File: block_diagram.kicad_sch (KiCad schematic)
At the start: 0 parts

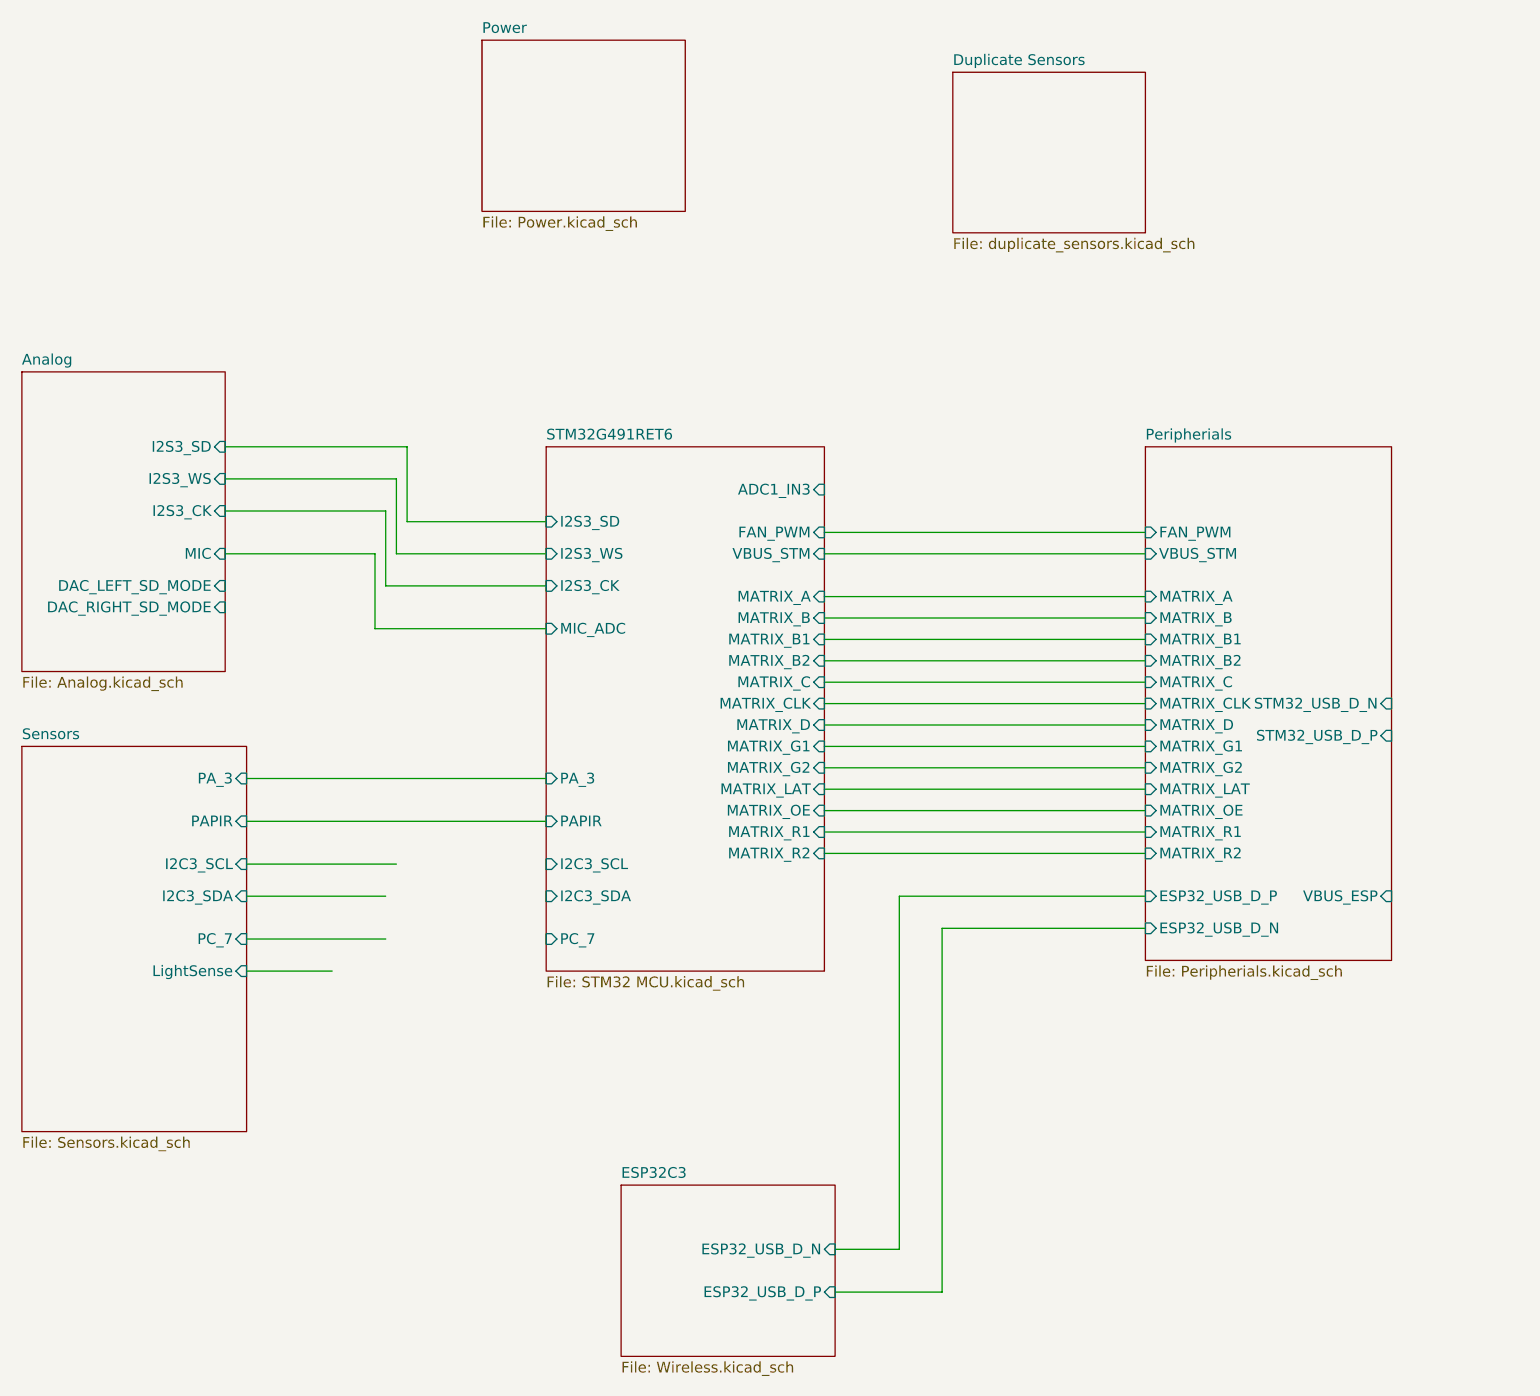
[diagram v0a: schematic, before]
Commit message: Major Changes - Schematic Done??
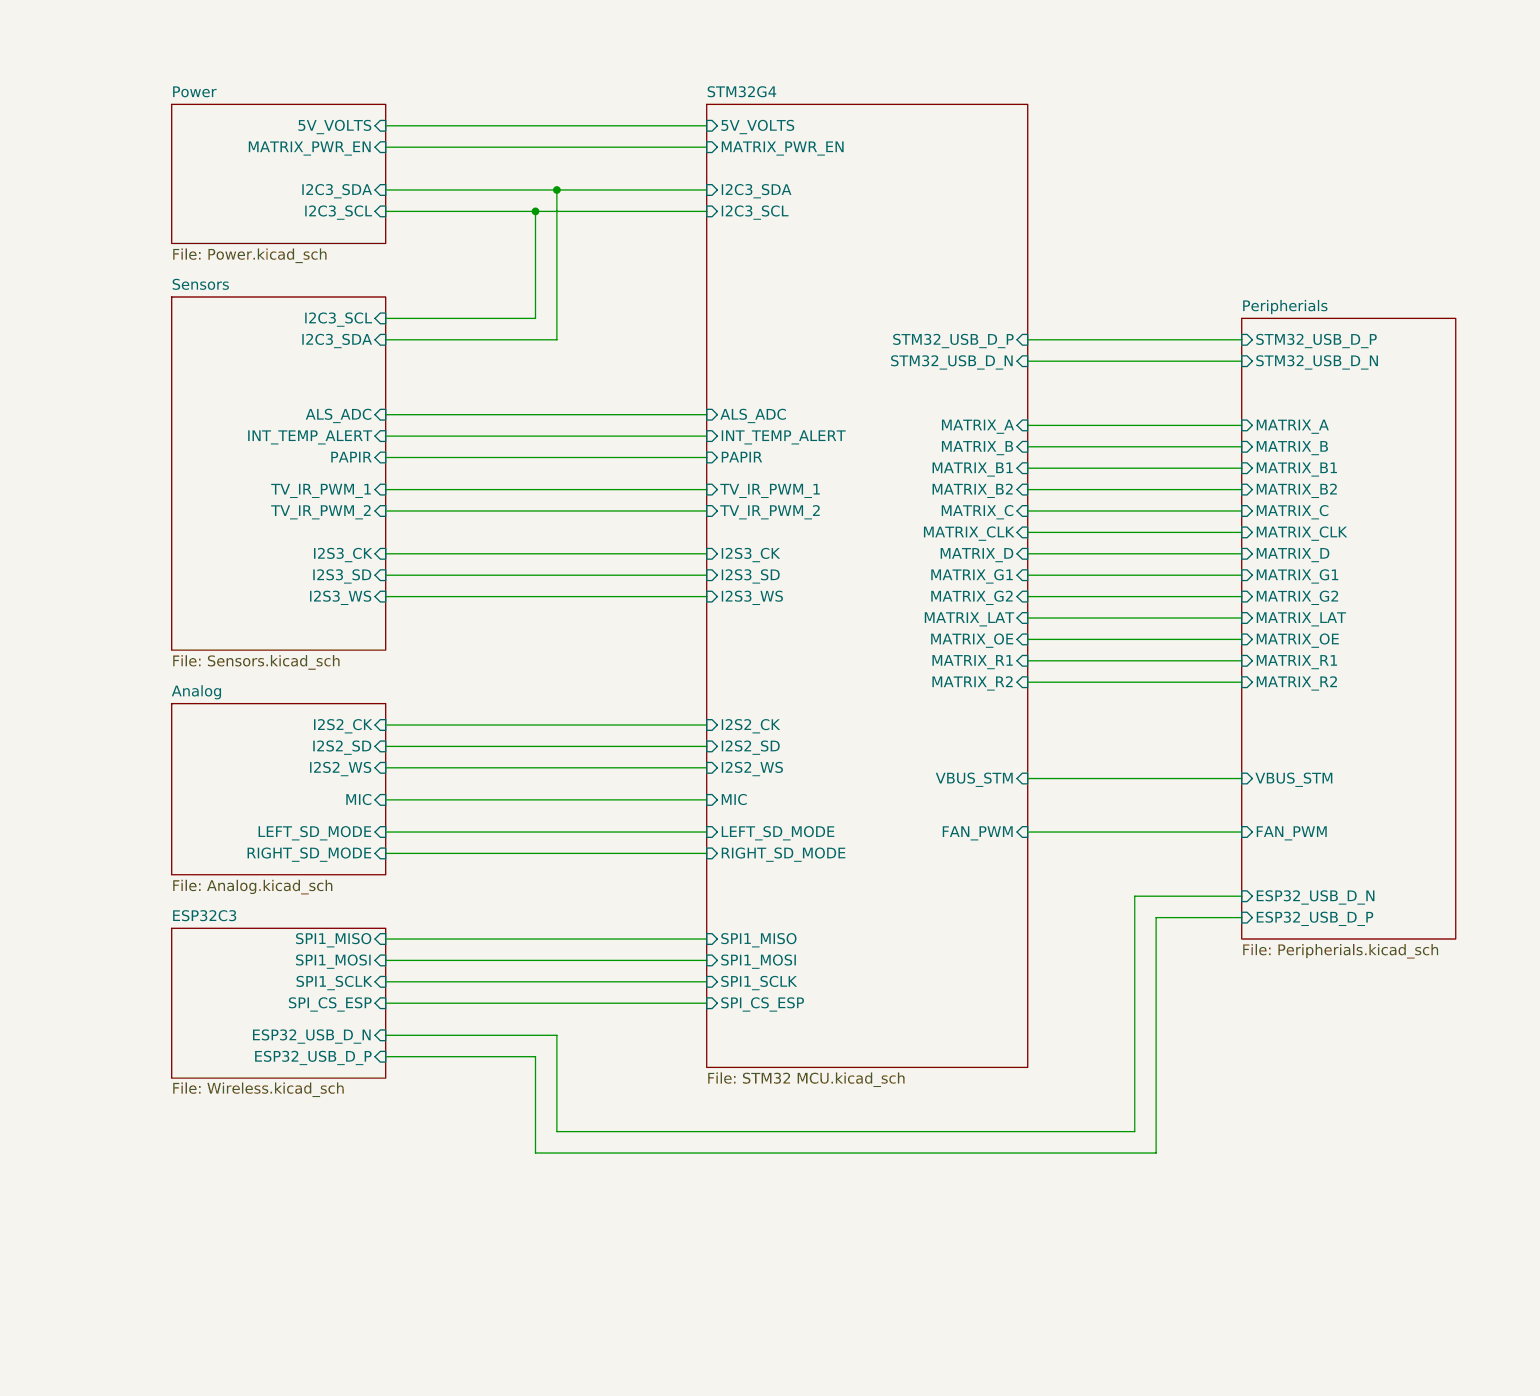
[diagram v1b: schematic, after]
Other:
- sheet STM32G491RET6 renamed STM32G4
- removed sheet Duplicate Sensors
- sheet Analog ports: added I2S2_CK, I2S2_SD, I2S2_WS, LEFT_SD_MODE, RIGHT_SD_MODE; removed DAC_LEFT_SD_MODE, DAC_RIGHT_SD_MODE, I2S3_CK, I2S3_SD, I2S3_WS
- sheet ESP32C3 ports: added SPI1_MISO, SPI1_MOSI, SPI1_SCLK, SPI_CS_ESP; removed none
- sheet Peripherials ports: added none; removed VBUS_ESP
- sheet Power ports: added 5V_VOLTS, I2C3_SCL, I2C3_SDA, MATRIX_PWR_EN; removed none
- sheet STM32G4 ports: added 5V_VOLTS, ALS_ADC, I2S2_CK, I2S2_SD, I2S2_WS, INT_TEMP_ALERT, LEFT_SD_MODE, MATRIX_PWR_EN, MIC, RIGHT_SD_MODE, SPI1_MISO, SPI1_MOSI, SPI1_SCLK, SPI_CS_ESP, STM32_USB_D_N, STM32_USB_D_P, TV_IR_PWM_1, TV_IR_PWM_2; removed ADC1_IN3, MIC_ADC, PA_3, PC_7
- sheet Sensors ports: added ALS_ADC, I2S3_CK, I2S3_SD, I2S3_WS, INT_TEMP_ALERT, TV_IR_PWM_1, TV_IR_PWM_2; removed LightSense, PA_3, PC_7
